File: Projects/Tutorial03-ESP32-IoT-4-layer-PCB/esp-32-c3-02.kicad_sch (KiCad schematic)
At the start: 11 parts, among them J3 GSD090012SEU, U3 ESP32-C3-WROOM-02-H4, U4 CP2102N-Axx-xQFN20, U5 USBLC6-2SC6, U6 W25Q32JVSSIQ

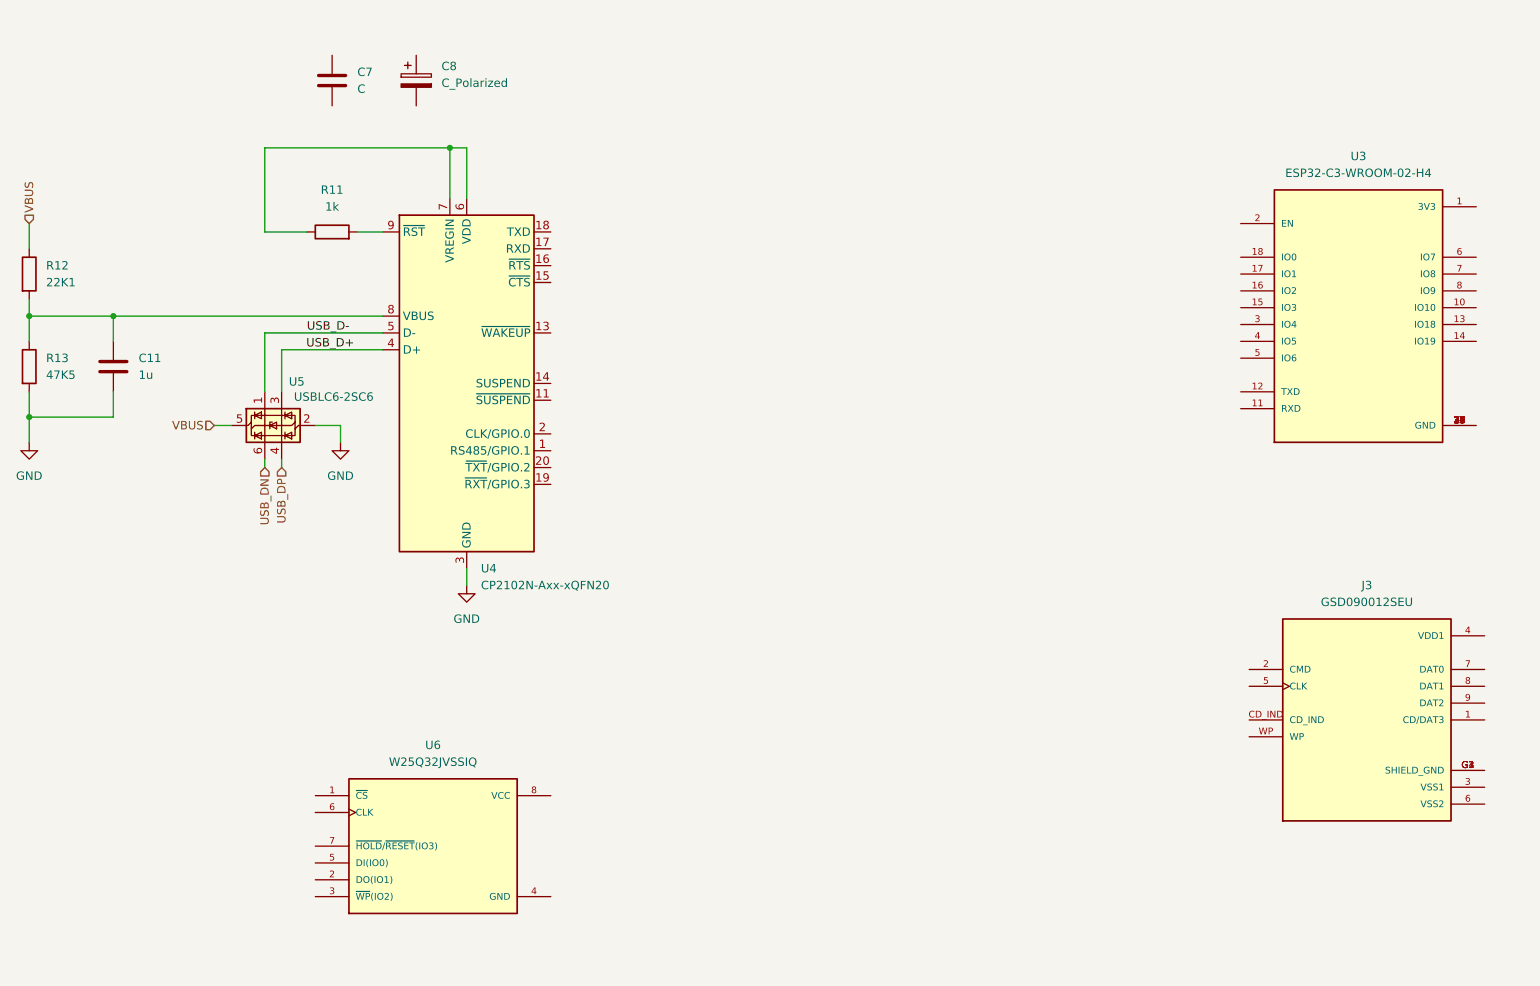
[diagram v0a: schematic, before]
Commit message: 20260301
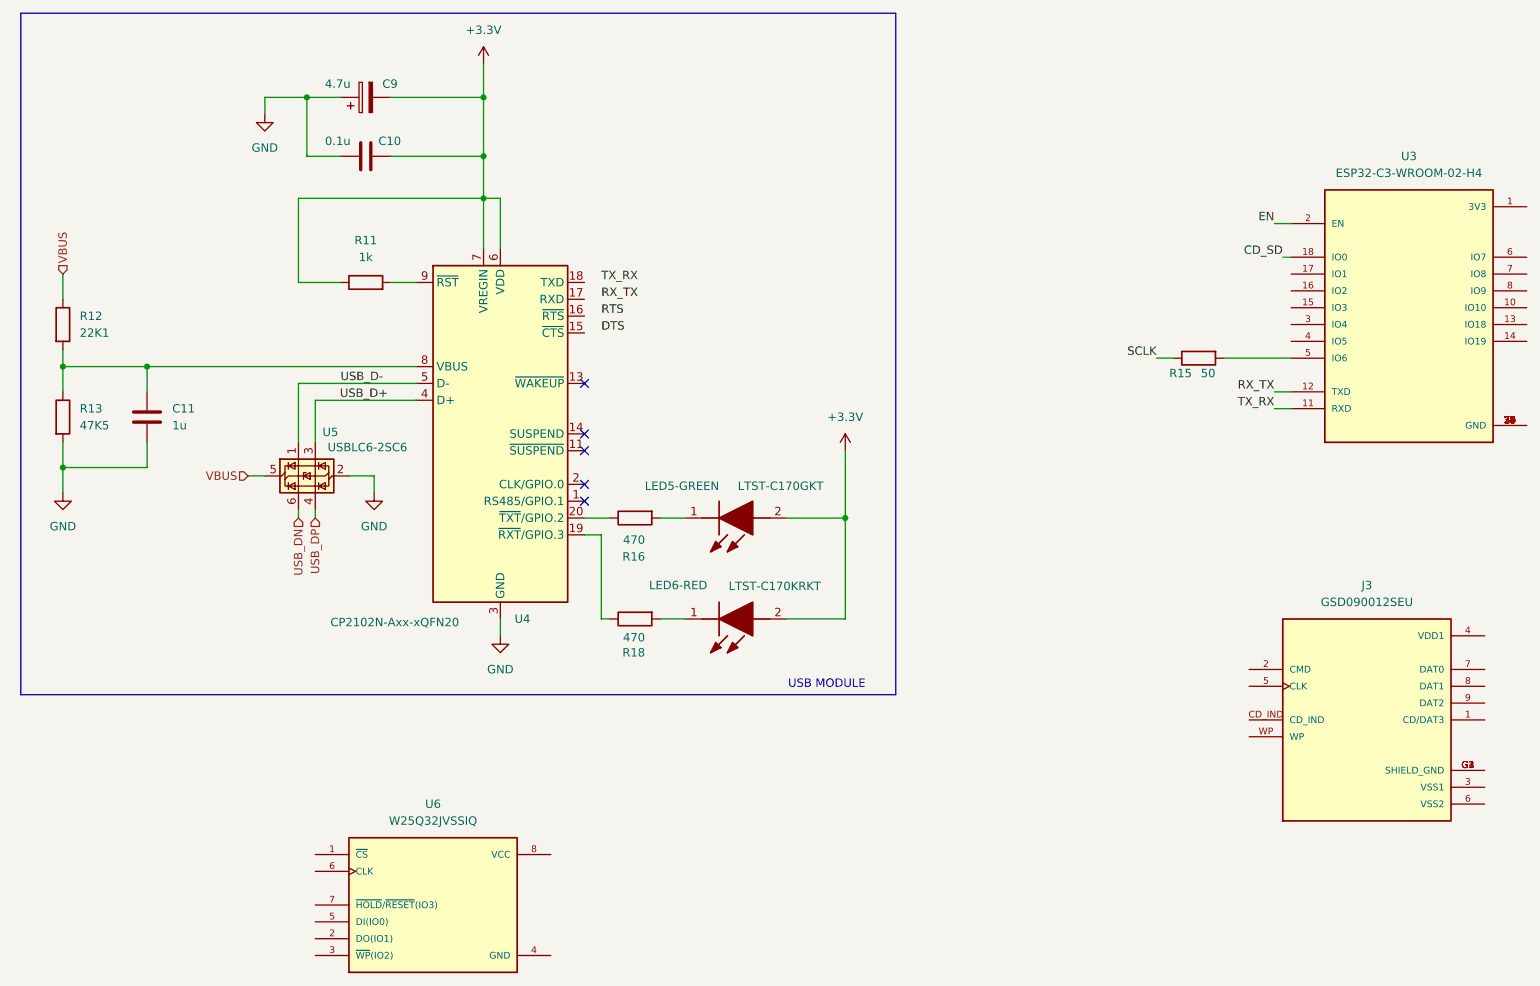
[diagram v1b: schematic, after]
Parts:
- added LED5-GREEN: LTST-C170GKT, LEDC2012X120N, symbol LTST-C170GKT:LTST-C170GKT
- added LED6-RED: LTST-C170KRKT, LEDC2012X120N, symbol LTST-C170KRKT:LTST-C170KRKT
- added R15: 50, symbol Device:R
- added R16, R18: 470, symbol Device:R
- C10: renamed from C7; value C -> 0.1u
- C9: renamed from C8; value C_Polarized -> 4.7u
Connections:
- net GND: now also C10.1, C9.1
- net +3.3V: now reaches R11.1, U4.6 (VDD), U4.7 (VREGIN)
- net +3.3V: now also C10.2, C9.2, LED5-GREEN.2 (A), LED6-RED.2 (A)
- net TX_RX: now reaches U3.11 (RXD)
- net RX_TX: now reaches U3.12 (TXD)
- net CD_SD: now reaches U3.18 (IO0)
- net EN: now reaches U3.2 (EN)
- net at U3.5 (IO6): now also R15.2
- net at U4.19 (~{RXT}/GPIO.3): now also R18.1
- net at U4.20 (~{TXT}/GPIO.2): now also R16.1
- new net: LED5-GREEN.1 (K), R16.2
- new net: LED6-RED.1 (K), R18.2
- new net SCLK: R15.1
- no-connect marks 0 -> 5
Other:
- note added: "USB MODULE"
- moved on the sheet: C10, C11, C9, R11, R12, R13, U3, U4, U5, U6
